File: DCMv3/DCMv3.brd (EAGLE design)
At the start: 160 x 100 mm, 27 parts, among them IC1 OKI-78SR-5_1.5-W36H-C, J1 DT15-12PA, J2 DTM15-12PA, M1 DRV8872DDA, Q1 IPD50P04P4L-11, U1 A000005, U2 TLE94108EL

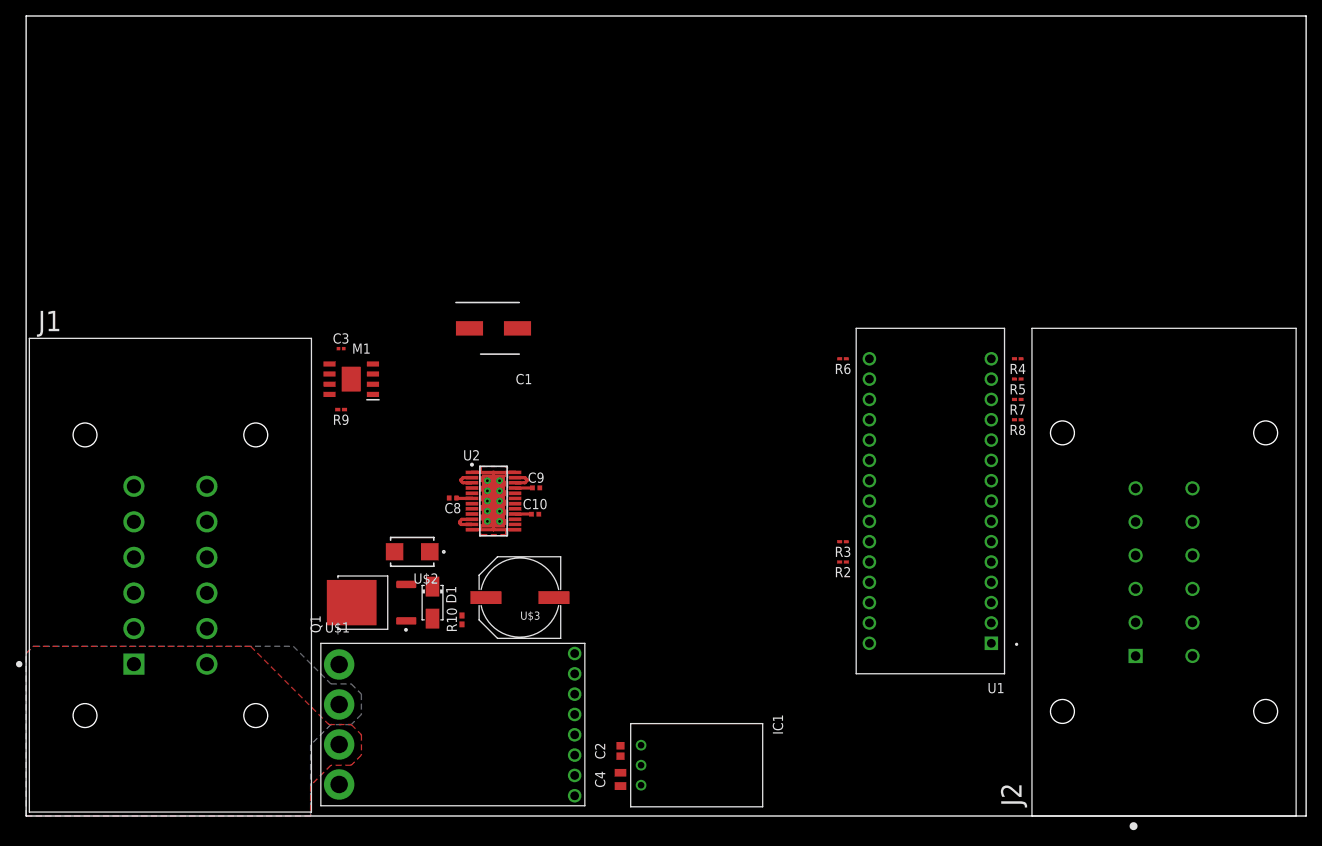
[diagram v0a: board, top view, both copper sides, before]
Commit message: updating DCMv3
x
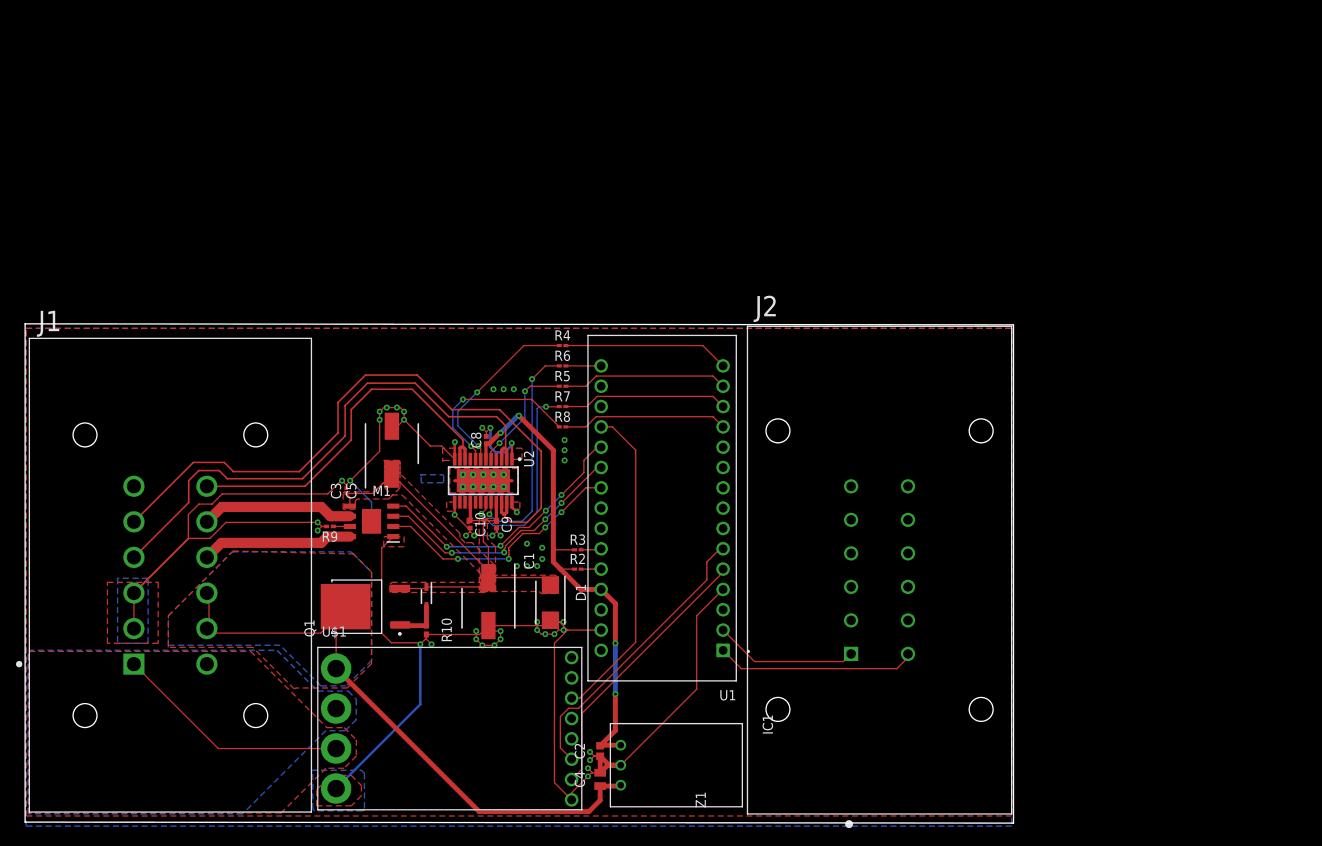
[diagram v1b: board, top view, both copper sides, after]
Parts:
- removed U$2: SM6T39A, SM6T39A:SM6T39A
- removed U$3: 47UF, EEE-FC1C471AP:CAPAE1030X1200
- added C5: EEE-FT1H470AP, SamacSys_Parts:CAPAE660X610N
- added Z1: MM3Z12VT1G, SamacSys_Parts:SOD2512X110N
- C1: value EEE-HDV470XAP -> EEE-FT1H470AP; device SamacSys_Parts:CAPAE645X770N -> SamacSys_Parts:CAPAE660X610N
- D1: value 1SMA5927BT3G -> SM6T39A; device 1sma59xx_10:DO214AC -> SamacSys_Parts:DIOM5436X265N
- moved R4 56.9 mm to (67.1, 58.8), turned to 0 degrees
- moved R5 56.9 mm to (67.1, 53.7), turned to 0 degrees
- moved R7 56.9 mm to (67.1, 51.2), turned to 0 degrees
- moved R8 56.9 mm to (67.1, 48.6), turned to 0 degrees
- moved J2 35.6 mm to (106.7, 30.7)
- moved R6 35.1 mm to (67.1, 56.3), turned to 0 degrees
- moved C1 34.2 mm to (57.8, 26.8), turned to 270 degrees
- moved U1 33.5 mm to (79.5, 38.5)
- moved R3 33.2 mm to (69.0, 33.3), turned to 0 degrees
- moved R2 33.2 mm to (69.0, 30.9), turned to 0 degrees
- moved M1 18.0 mm to (43.2, 36.8)
- moved C3 17.8 mm to (40.0, 40.6), turned to 90 degrees
- moved D1 14.7 mm to (65.5, 26.7)
- moved R9 14.7 mm to (38.0, 36.2), turned to 180 degrees
- moved C8 8.36 mm to (57.5, 47.0), turned to 90 degrees
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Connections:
- removed net MIR_SEL: R3.2, U1.25
- removed net N$18: U1.20
- removed net P_WIN: U1.22
- new net N$6: J2.6
- new net N$7: J2.7
- net FOLD_A: now also J1.8
- net FOLD_B: now also J1.9
- net GATE: now also Z1.2; no longer D1.A
- net GND: now also C5.2, D1.2, J1.2, J1.3; no longer J1.6, U$2.A, U$3.-
- net ILLUM_IN: now also R3.2, U1.25; no longer U1.21
- net IN1: now also U1.21
- net IN2: now also U1.22
- net MIR_COM: now also J1.5
- net MIR_H: now also J1.4
- net MIR_V: now also J1.7
- net N$10: now also J2.10; no longer J1.10
- net N$13: now also J2.11; no longer J1.11
- net N$2: now also J2.2; no longer J1.2
- net N$3: now also J2.3; no longer J1.3
- net N$4: now also J2.4; no longer J1.4
- net N$5: now also J2.5; no longer J1.5
- net N$8: now also J2.8; no longer J1.8
- net N$9: now also J2.9; no longer J1.9
- net NFAULT: now also U1.20
- net RX: now also J2.1
- net TX: now also J2.12
- net VBAT: now also J1.10, J1.11; no longer J1.7
- net VS: now also C5.1, D1.1, Z1.1; no longer D1.C, U$2.C, U$3.+
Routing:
- net GND: track 28.5 -> 291.3 mm, vias 0 -> 50
- net MIR_COM: track 3.33 -> 82.0 mm
- net VBAT: track 0.00 -> 74.9 mm
- net MIR_H: track 3.08 -> 68.2 mm
- net 5V: track 1.95 -> 63.0 mm, vias 0 -> 4
- net VS: track 4.26 -> 61.7 mm
- net MIR_V: track 3.41 -> 46.2 mm
- net CS: track 0.00 -> 40.4 mm
- net PWM: track 0.00 -> 36.3 mm
- net NFAULT: track 0.00 -> 34.1 mm, vias 0 -> 4
- net DIR: track 0.00 -> 34.1 mm
- net IN1: track 0.00 -> 32.7 mm, vias 0 -> 4
- net IN2: track 0.00 -> 32.2 mm, vias 0 -> 4
- net WIN_B: track 0.00 -> 29.6 mm
- net SCK: track 0.00 -> 28.4 mm, vias 0 -> 2
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- added copper zone on layer 1, net VBAT
- added copper zone on layer 16, net VBAT
- added copper zone on layer 1, net VS
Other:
- board size 160 x 100 mm -> 123.6 x 62.4 mm
